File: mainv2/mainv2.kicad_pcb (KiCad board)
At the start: 4 copper layers, 57.2 x 53 mm, 46 parts, among them IC1 SPX3819M5-L-3-3_TR, IC3 AT45DB081E-SSHN-B, J1 12401948E412A, J2 Conn_01x02_Pin, J4 SAMTEC-FTS-107-03-X-D, Q1 PMOS, U1 ESP32-C6, U2 MCP73831-2-OT, Y2 ECS-400-10-37B-CKY-TR3

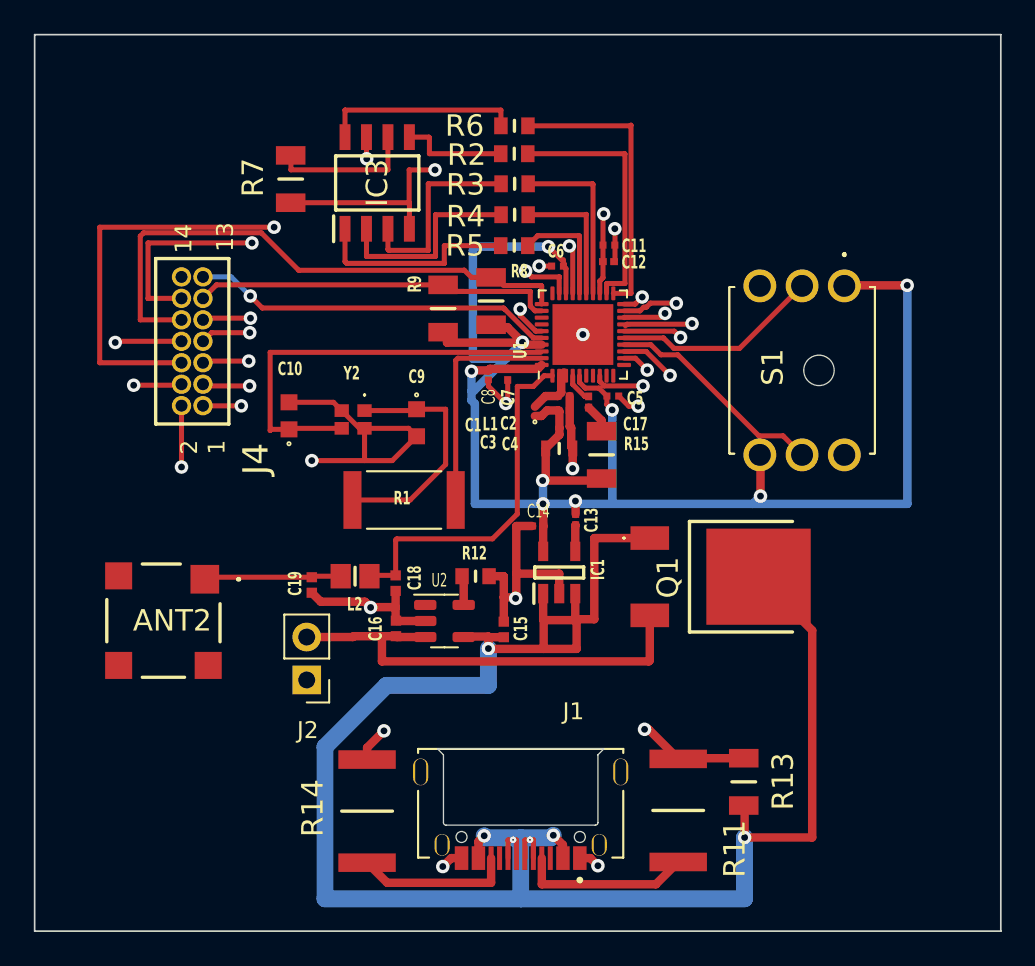
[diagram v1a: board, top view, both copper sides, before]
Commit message: Board Update
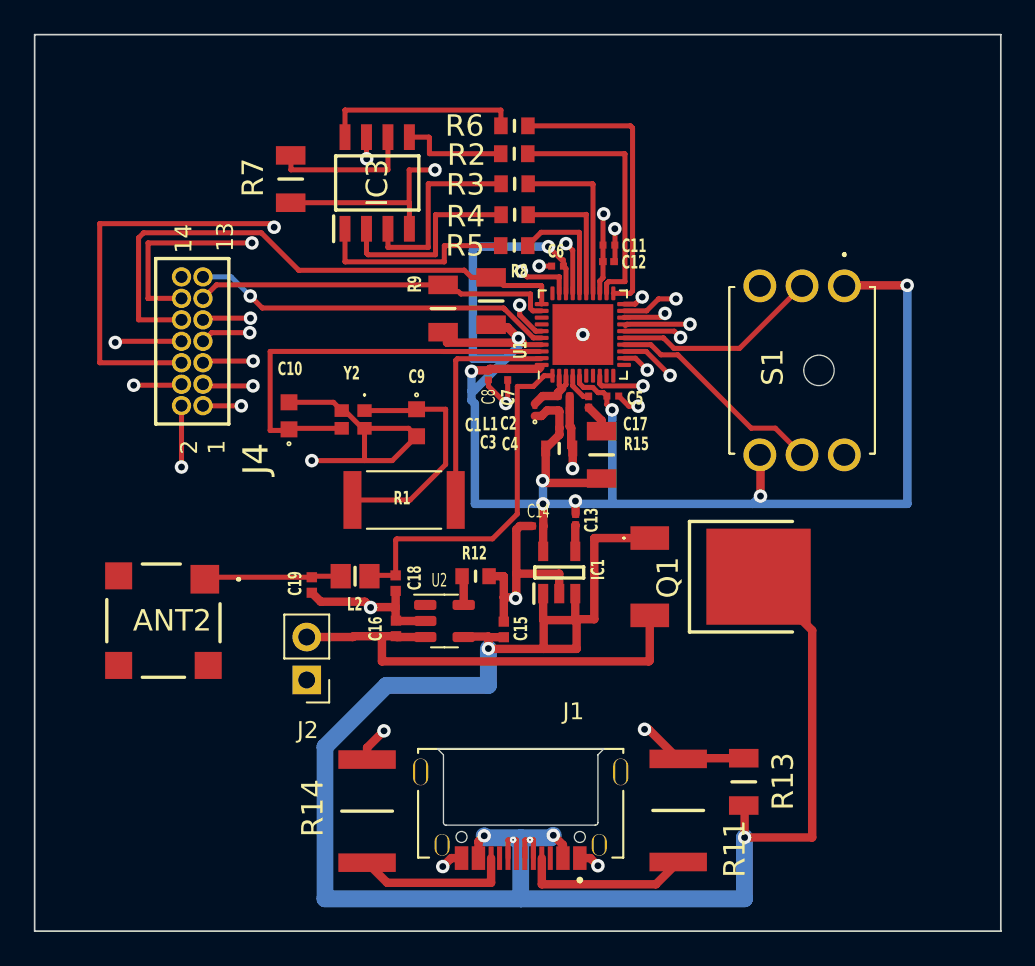
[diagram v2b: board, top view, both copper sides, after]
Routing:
- net +3.3V: track 109.1 -> 110.6 mm
- net /I2CEXT0_SCL_in: track 32.7 -> 33.7 mm
- net Net-(C1-Pad1): track 3.17 -> 3.94 mm
